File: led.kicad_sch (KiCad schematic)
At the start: 19 parts, among them U8 T8Q144xx

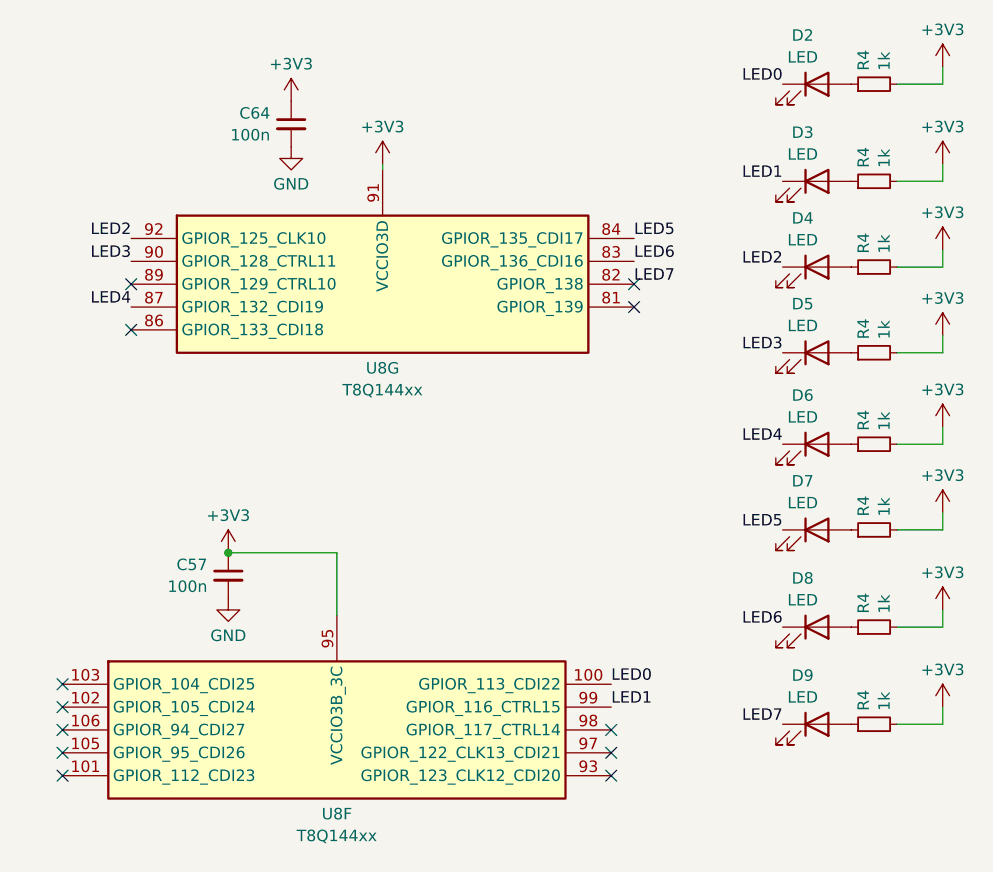
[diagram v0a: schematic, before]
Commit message: sdram layout done - COMPLETE REWORK NEEDED
cannot mix LVDS and GPIO banks due to too different timing
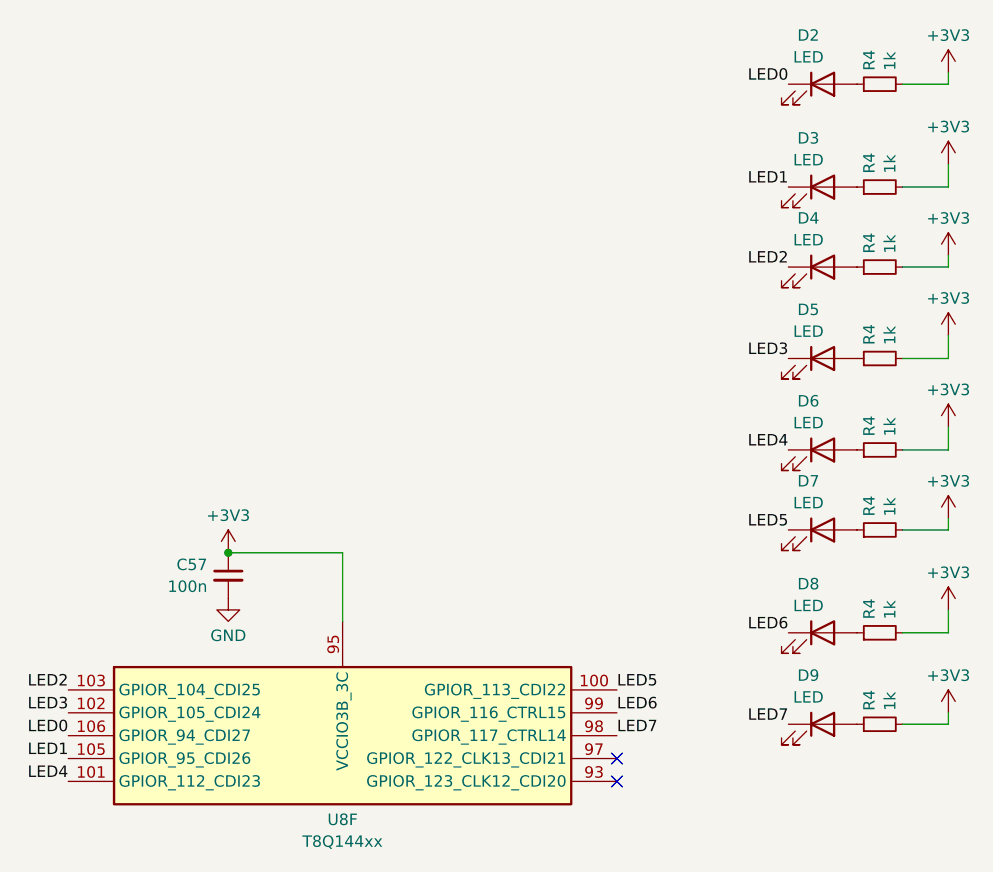
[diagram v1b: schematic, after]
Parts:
- removed C64: 100n, Capacitor_SMD:C_0603_1608Metric, symbol Device:C_Small
- removed unit 7 of U8
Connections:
- net LED0: now also U8.106 (GPIOR_94_CDI27); no longer U8.100 (GPIOR_113_CDI22)
- net LED1: now also U8.105 (GPIOR_95_CDI26); no longer U8.99 (GPIOR_116_CTRL15)
- net LED2: now also U8.103 (GPIOR_104_CDI25)
- net LED3: now also U8.102 (GPIOR_105_CDI24)
- net LED4: now also U8.101 (GPIOR_112_CDI23)
- net LED5: now also U8.100 (GPIOR_113_CDI22)
- net LED6: now also U8.99 (GPIOR_116_CTRL15)
- net LED7: now also U8.98 (GPIOR_117_CTRL14)
- no-connect marks 12 -> 2
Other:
- moved on the sheet: D2, D3, D4, D5, D6, D7, D8, D9, R4, U8F
